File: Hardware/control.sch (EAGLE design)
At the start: 14 parts, among them IC1 317T

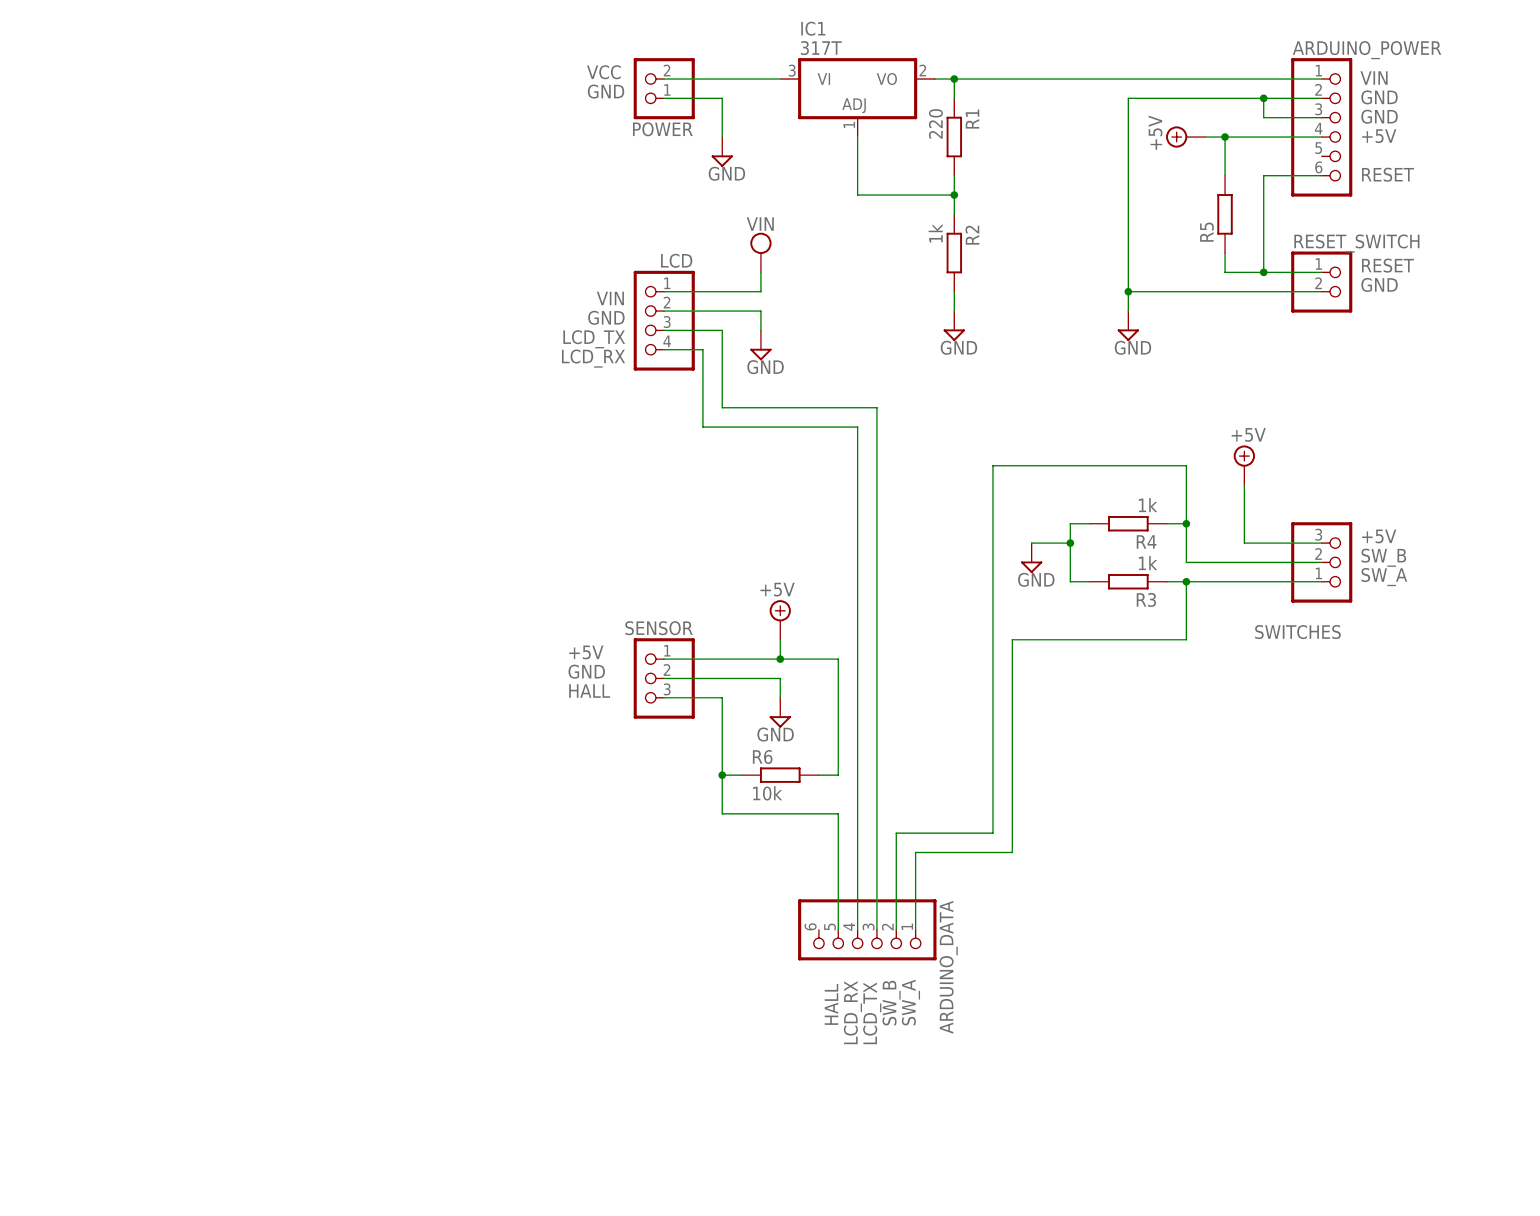
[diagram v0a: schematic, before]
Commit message: Added some screenshots ready for blogging
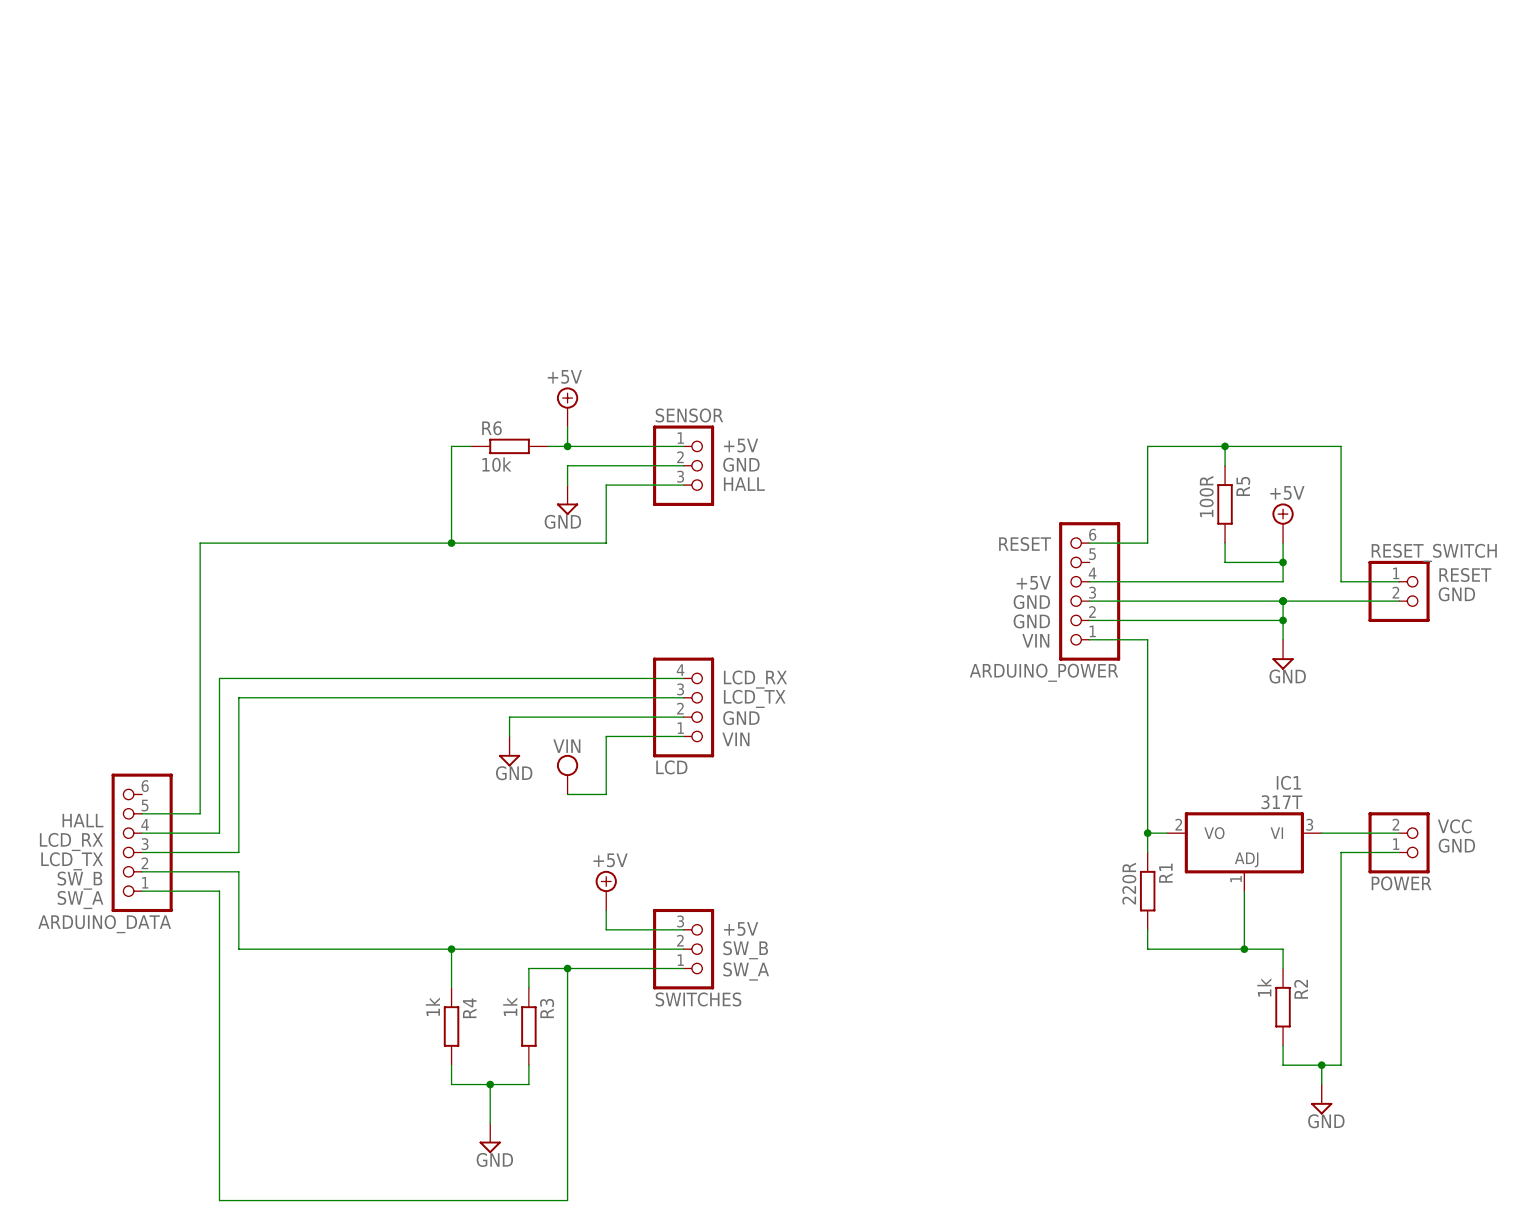
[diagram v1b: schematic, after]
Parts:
- R1: value 220 -> 220R
- R5: value (none) -> 100R
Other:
- moved on the sheet: ARDUINO_DATA, ARDUINO_POWER, IC1, LCD, POWER, R1, R2, R3, R4, R5, R6, RESET_SWITCH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
